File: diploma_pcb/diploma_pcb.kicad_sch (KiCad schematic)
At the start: 17 parts, among them Q1 2SC3356, Q3 2SC3356

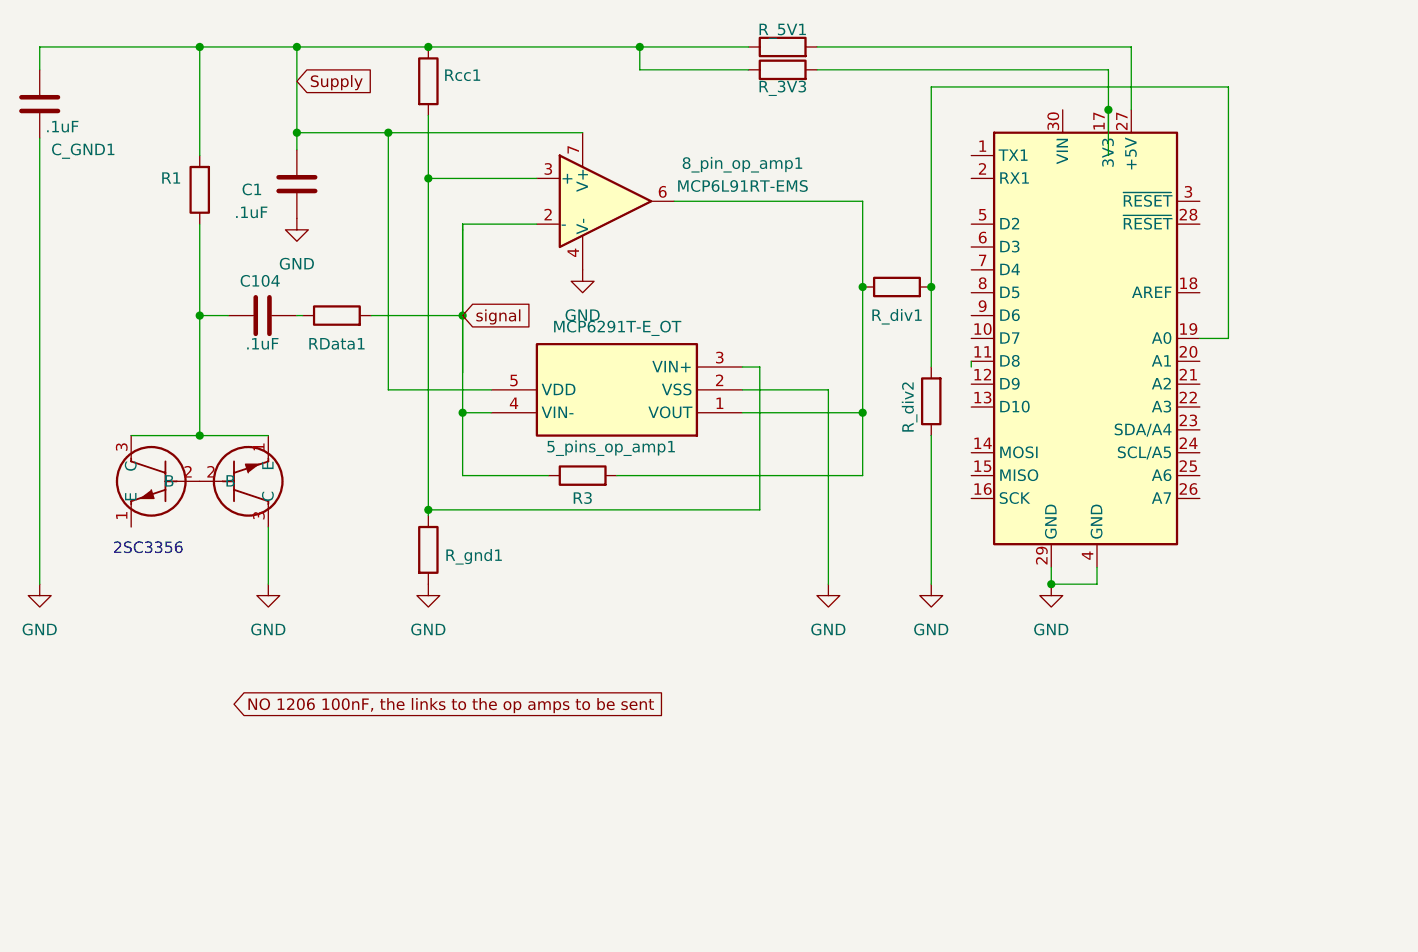
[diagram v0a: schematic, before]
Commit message: rgb placed
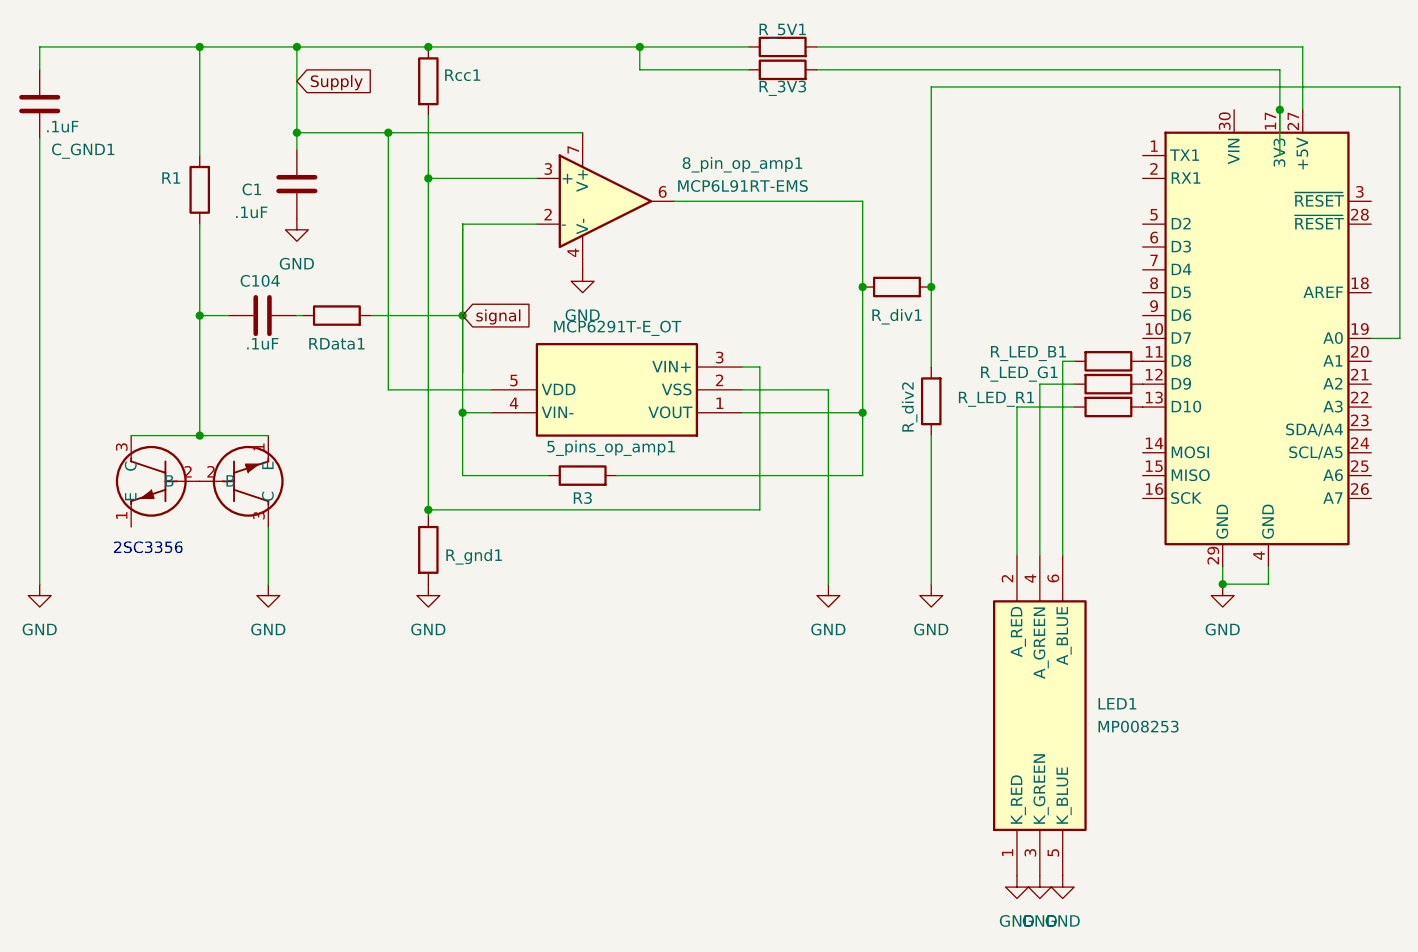
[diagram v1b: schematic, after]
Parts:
- added LED1: MP008253, MP008253:MP008253, symbol MP008253:MP008253
- added R_LED_B1, R_LED_G1, R_LED_R1: R, Resistor_SMD:R_1206_3216Metric, symbol Device:R
- R1, R3, RData1, R_3V3, R_5V1, R_div1, R_div2, R_gnd1, Rcc1: footprint 1206:RESC3116X65N -> Resistor_SMD:R_1206_3216Metric
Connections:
- net GND: now also LED1.1 (K_RED), LED1.3 (K_GREEN), LED1.5 (K_BLUE)
- net at A1.11 (D8): now also R_LED_B1.1
- net at A1.12 (D9): now also R_LED_G1.1
- net at A1.13 (D10): now also R_LED_R1.1
- new net: LED1.2 (A_RED), R_LED_R1.2
- new net: LED1.4 (A_GREEN), R_LED_G1.2
- new net: LED1.6 (A_BLUE), R_LED_B1.2
